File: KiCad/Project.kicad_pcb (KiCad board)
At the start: 2 copper layers, 70 x 40.6 mm, 55 parts, among them J2 Power & Output Test Points, J3 Inputs Test Points, Q1 BUK9832-55A, Q2 BUK9832-55A, Q3 BUK9832-55A, SW1 Power, SW2 Fire, SW3 Freq Select, SW4 Fire Select, U1 TLV1117-50, U2 PIC16F1788-IP, U3 Audio Board

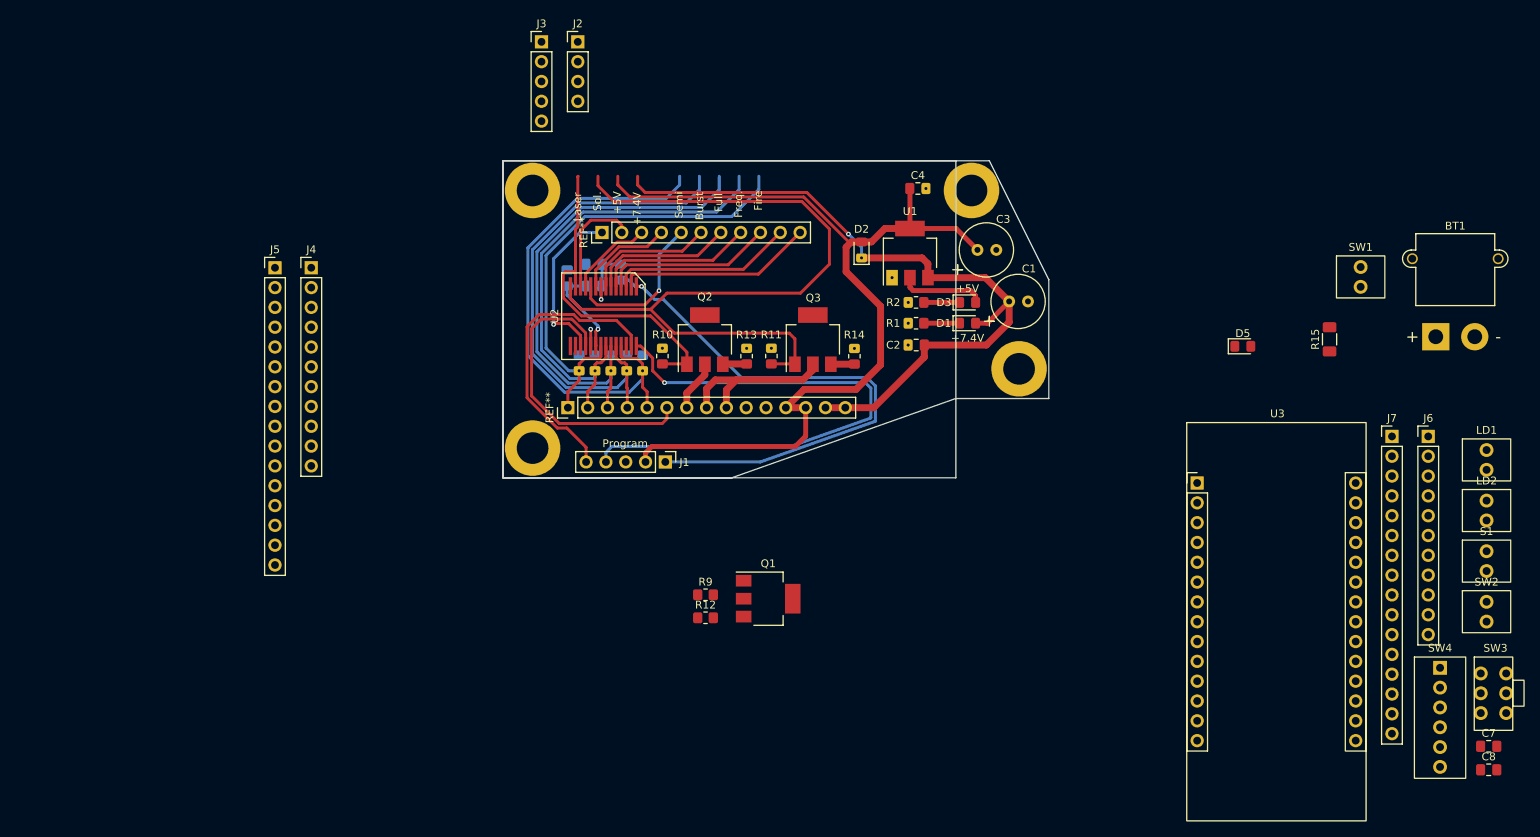
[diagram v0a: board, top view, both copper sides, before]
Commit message: PCB nearly done for the blaster
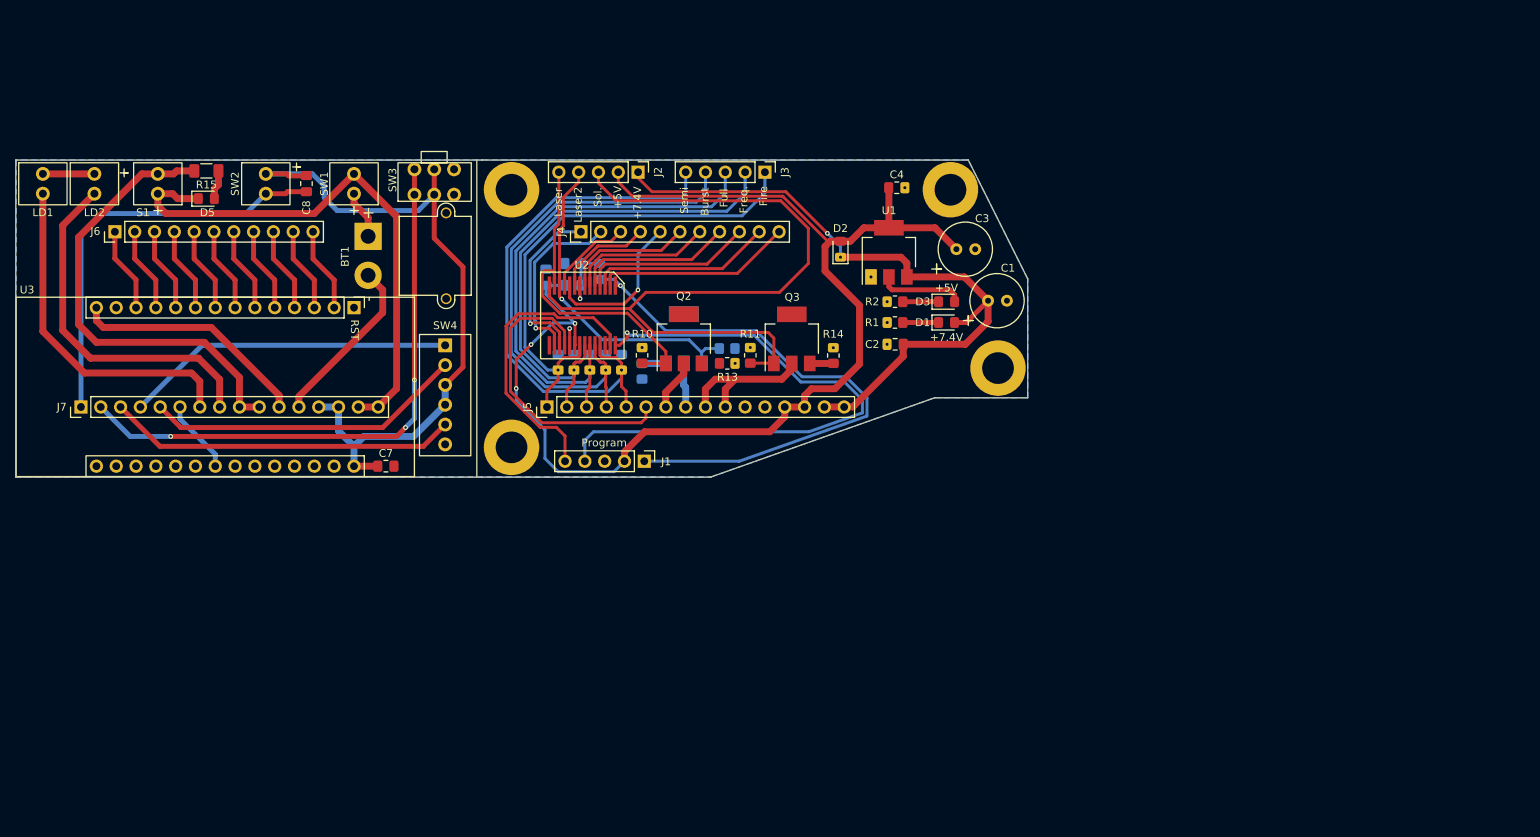
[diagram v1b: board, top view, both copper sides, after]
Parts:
- removed the REF** at (87.4, 82.0)
- removed the REF** at (91.7, 59.6)
- J2: footprint Connector_PinHeader_2.54mm:PinHeader_1x04_P2.54mm_Vertical -> Connector_PinHeader_2.54mm:PinHeader_1x05_P2.54mm_Vertical
- Q1, R12, R9: moved to B.Cu
- moved LD1 188.4 mm to (20.1, 52.1)
- moved LD2 183.3 mm to (26.7, 52.1)
- moved S1 176.4 mm to (34.8, 54.6), turned to 180 degrees
- moved J6 170.4 mm to (29.3, 59.5), turned to 90 degrees
- moved C8 169.1 mm to (53.8, 53.3), turned to -90 degrees
- moved J7 168.1 mm to (24.9, 81.9), turned to 90 degrees
- moved SW2 165.8 mm to (48.6, 52.1)
- moved SW3 149.8 mm to (67.7, 54.7), turned to 90 degrees
- moved C7 145.9 mm to (64.0, 89.5), turned to 180 degrees
- moved R15 145.6 mm to (41.0, 51.7), turned to 0 degrees
- moved D5 134.2 mm to (41.0, 55.2)
- moved SW4 134.1 mm to (71.6, 74.0)
- moved SW1 129.4 mm to (59.9, 54.6), turned to 180 degrees
- moved BT1 125.7 mm to (75.5, 62.6), turned to -90 degrees
- moved U3 110.4 mm to (59.9, 69.2), turned to -90 degrees
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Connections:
- C3 pad 1: +5V_Top -> +5V
- C4 pad 1: +5V_Top -> +5V
- C5 pad 2: Net-(C5-Pad2) -> GND
- C6 pad 1: Net-(C6-Pad1) -> GND
- C6 pad 2: +5V_Top -> +5V
- C7 pad 1: Net-(C7-Pad1) -> GND
- D2 pad 2: +5V_Top -> +5V
- D3 pad 2: +5V_Top -> +5V
- J1 pad 2: +5V_Top -> +5V
- J1 pad 3: Net-(J1-Pad3) -> GND
- J2 pad 2: +5V_Top -> +5V
- J2 pad 3: Laser/PWM -> Net-(Q3-G)
- J2 pad 4: Solenoid -> Net-(Q1-G)
- J5 pad 11: Net-(J5-Pad11) -> GND
- J5 pad 12: Net-(J5-Pad11) -> GND
- J5 pad 13: +5V_Top -> +5V
- J5 pad 14: +5V_Top -> +5V
- J7 pad 11: Net-(J7-Pad11) -> GND
- J7 pad 12: Net-(J7-Pad11) -> GND
- R10 pad 2: Net-(R10-Pad2) -> GND
- R11 pad 2: Net-(R11-Pad2) -> GND
- R12 pad 2: Net-(R12-Pad2) -> GND
- R13 pad 2: Net-(R13-Pad2) -> GND
- R14 pad 2: Net-(R14-Pad2) -> GND
- R3 pad 2: +5V_Top -> +5V
- R4 pad 2: Net-(R4-Pad2) -> GND
- R5 pad 2: Net-(R4-Pad2) -> GND
- R6 pad 2: Net-(R4-Pad2) -> GND
- R7 pad 2: Net-(R4-Pad2) -> GND
- R8 pad 2: Net-(R4-Pad2) -> GND
- R9 pad 2: Net-(R9-Pad2) -> GND
- U1 pad 2: +5V_Top -> +5V
- U2 pad 20: +5V_Top -> +5V
- U3 pad 14: Net-(U3-GND-Pad14) -> GND
- U3 pad 15: Net-(U3-GND-Pad14) -> GND
- U3 pad 18: Net-(U3-GND-Pad14) -> GND
- U3 pad 27: Net-(U3-GND-Pad14) -> GND
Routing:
- net Net-(D1-K): track 98.5 -> 4.59 mm, vias 1 -> 0
- net +7.4V: track 0.00 -> 88.6 mm, vias 0 -> 1
- net Frequency Select_Top: track 0.00 -> 74.8 mm, vias 0 -> 3
- net +5V_Top: track 23.4 -> 97.7 mm, vias 1 -> 0
- net Semi-Auto: track 0.00 -> 71.0 mm
- net +7.4V_Top: track 0.00 -> 70.3 mm
- net Burst: track 0.00 -> 67.9 mm
- net Net-(U2-P1D/AN11/RB4): track 66.4 -> 0.00 mm
- net Full-Auto: track 0.00 -> 65.9 mm
- net Frequency Select: track 0.00 -> 65.4 mm
- net Fire: track 0.00 -> 64.8 mm
- net Net-(U2-PGM/C12IN2-/AN8/RB3): track 63.7 -> 0.00 mm
- net Net-(U2-P1B/AN8/RB2): track 61.7 -> 0.00 mm
- net Net-(SW3-A): track 61.2 -> 0.00 mm
- net Net-(U2-INT/AN12/RB0): track 60.5 -> 0.00 mm
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- added copper zone on B.Cu, net GND
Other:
- board size 70 x 40.6 mm -> 129.7 x 40.6 mm
- board text added: "Laser2"
- board text added: "RST"
